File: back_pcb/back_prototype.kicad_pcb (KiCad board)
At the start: 2 copper layers, 40 x 100 mm, 358 parts

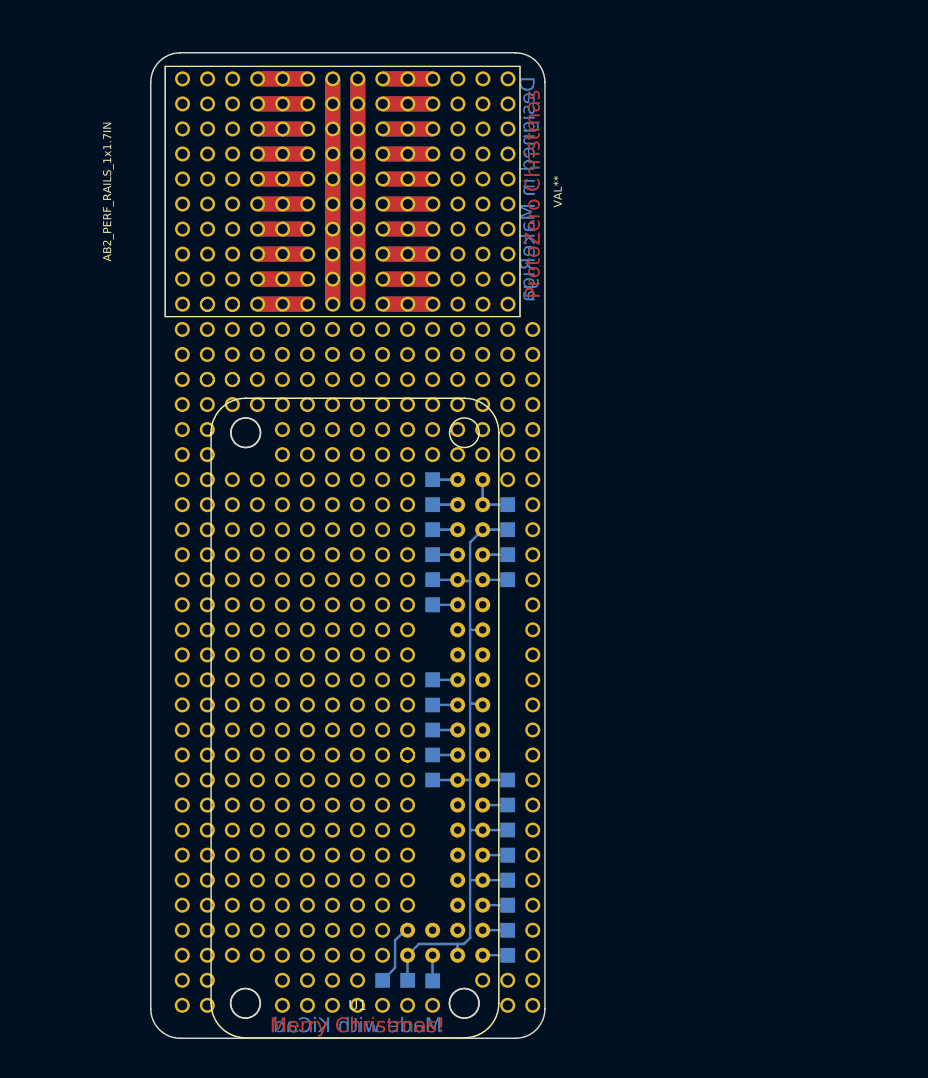
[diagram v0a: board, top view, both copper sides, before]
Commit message: Started new back PCB
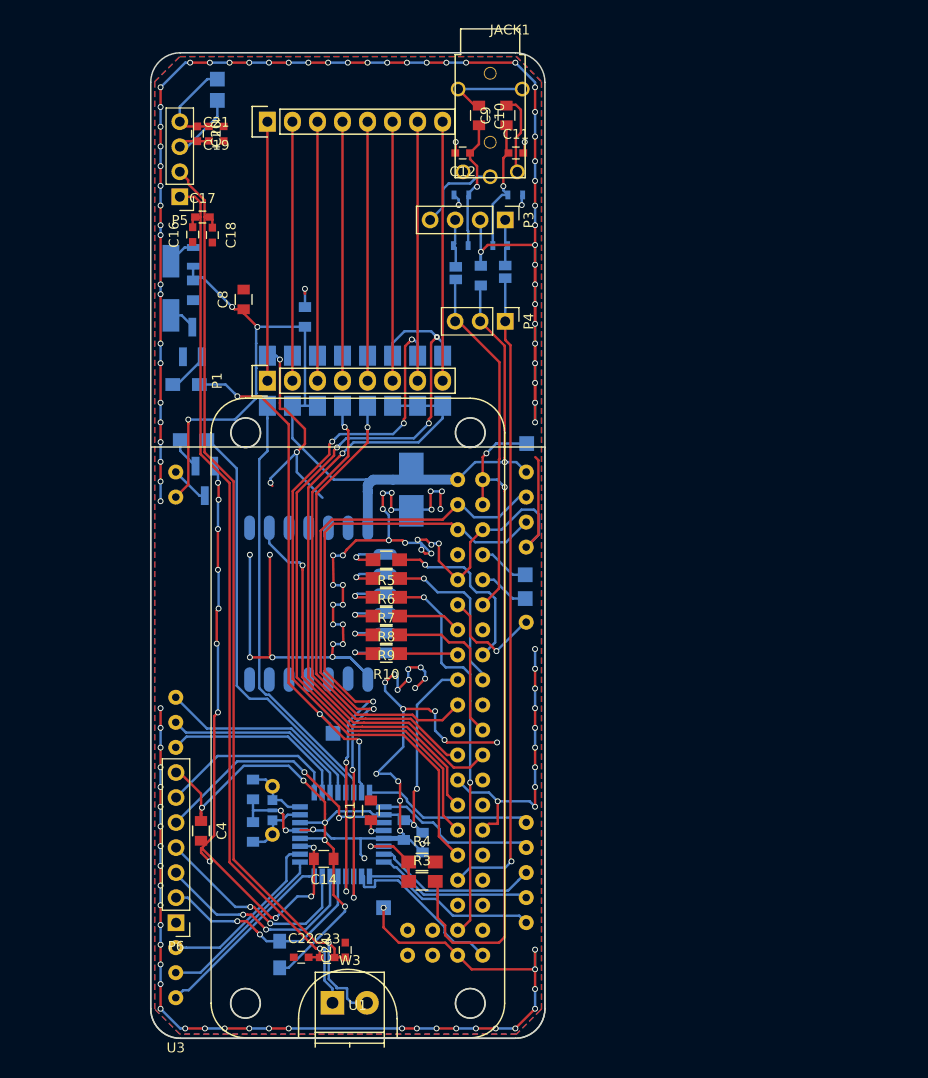
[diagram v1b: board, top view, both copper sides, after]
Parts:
- removed ? (x330): , single_proto_pad:PROTO_PAD
- removed AB2_PERF_RAILS_1x1.7IN: VAL**, prototyping_area_10x14:PROTO_AREA_10x14
- removed W10: RXD, Measurement_Points:Measurement_Point_Square-SMD-Pad_Small
- removed W13: SDA, Measurement_Points:Measurement_Point_Square-SMD-Pad_Small
- removed W14: SCL, Measurement_Points:Measurement_Point_Square-SMD-Pad_Small
- removed W15: MOSI, Measurement_Points:Measurement_Point_Square-SMD-Pad_Small
- removed W16: MISO, Measurement_Points:Measurement_Point_Square-SMD-Pad_Small
- removed W17: SCK, Measurement_Points:Measurement_Point_Square-SMD-Pad_Small
- removed W18: , Measurement_Points:Measurement_Point_Square-SMD-Pad_Small
- removed W19: CS1, Measurement_Points:Measurement_Point_Square-SMD-Pad_Small
- removed W20: GP4, Measurement_Points:Measurement_Point_Square-SMD-Pad_Small
- removed W21: GP17, Measurement_Points:Measurement_Point_Square-SMD-Pad_Small
- removed W22: GP12, Measurement_Points:Measurement_Point_Square-SMD-Pad_Small
- removed W23: GP16, Measurement_Points:Measurement_Point_Square-SMD-Pad_Small
- removed W24: GP20, Measurement_Points:Measurement_Point_Square-SMD-Pad_Small
- removed W25: GP21, Measurement_Points:Measurement_Point_Square-SMD-Pad_Small
- removed W26, W6, W8: GND, Measurement_Points:Measurement_Point_Square-SMD-Pad_Small
- removed W9: TXD, Measurement_Points:Measurement_Point_Square-SMD-Pad_Small
- added C1: C_Small, Capacitors_SMD:C_0805, F.Cu at (63.8, 116.9)
- added C10: C_Small, Capacitors_SMD:C_0805, F.Cu at (74.8, 46.4)
- added C11: C_Small, Capacitors_SMD:C_0603, F.Cu at (78.5, 50.2)
- added C12: C, Capacitors_SMD:C_0603, F.Cu at (73.2, 50.2)
- added C13: C_Small, Capacitors_SMD:C_0805, B.Cu at (75.0, 62.6)
- added C14: C_Small, Capacitors_SMD:C_0805, F.Cu at (59.1, 121.8)
- added C15: C_Small, Capacitors_Tantalum_SMD:CP_Tantalum_Case-B_EIA-3528-21_Hand, B.Cu at (67.9, 84.3)
- added C16: C_Small, Capacitors_SMD:C_0603, F.Cu at (45.8, 58.4)
- added C17: C_Small, Capacitors_SMD:C_0603, F.Cu at (46.7, 56.7)
- added C18: C_Small, Capacitors_SMD:C_0603, F.Cu at (47.8, 58.5)
- added C19: C_Small, Capacitors_SMD:C_0603, F.Cu at (48.1, 47.5)
- added C2: C_Small, Capacitors_SMD:C_0805, B.Cu at (51.9, 119.1)
- added C20: C_Small, Capacitors_SMD:C_0603, F.Cu at (46.2, 48.2)
- added C21: C_Small, Capacitors_SMD:C_0603, F.Cu at (48.1, 48.9)
- added C22: C_Small, Capacitors_SMD:C_0603, F.Cu at (56.8, 131.8)
- added C23: C_Small, Capacitors_SMD:C_0603, F.Cu at (59.4, 131.8)
- added C24: C_Small, Capacitors_SMD:C_0603, F.Cu at (61.2, 131.0)
- added C25: C_Small, Capacitors_SMD:C_0805, B.Cu at (45.8, 64.1)
- added C3: C_Small, Capacitors_SMD:C_0805, B.Cu at (51.9, 114.7)
- added C4: C_Small, Capacitors_SMD:C_0805, F.Cu at (46.6, 119.0)
- added C5: C_Small, Capacitors_SMD:C_0805, B.Cu at (67.2, 118.9)
- added C6: C_Small, Capacitors_SMD:C_0805, B.Cu at (57.1, 66.8)
- added C7: C_Small, Capacitors_SMD:C_0805, B.Cu at (69.1, 120.1)
- added C8: C_Small, Capacitors_SMD:C_0805, F.Cu at (50.9, 65.0)
- added C9: C, Capacitors_SMD:C_0805, F.Cu at (77.6, 46.4)
- added D1: D, Diodes_SMD:MiniMELF_Handsoldering, B.Cu at (43.5, 63.9)
- added IC1: ATMEGA328P-A, Housings_QFP:TQFP-32_7x7mm_Pitch0.8mm, B.Cu at (60.9, 119.3)
- added JACK1: AB2_JACK_3.5MM-4P, footprints:4P_RPi_AV_jack, F.Cu at (75.9, 52.6)
- added JP1: JUMPER, Connect:GS2, B.Cu at (77.5, 62.2)
- added JP2: JUMPER, Connect:GS2, B.Cu at (72.5, 62.4)
- added P1: SwitchableHeader-3x08, switchable_header:Pin_Header_Straight_1x08, F.Cu at (53.3, 73.3)
- added P2: CONN_01X08, Pin_Headers:Pin_Header_Straight_1x08, F.Cu at (53.3, 47.0)
- added P3: CONN_01X04, Pin_Headers:Pin_Header_Straight_1x04_Pitch2.54mm, F.Cu at (77.5, 57.0)
- added P4: CONN_01X03, Pin_Headers:Pin_Header_Straight_1x03_Pitch2.54mm, F.Cu at (77.5, 67.2)
- added P5: CONN_01X04, Pin_Headers:Pin_Header_Straight_1x04_Pitch2.54mm, F.Cu at (44.5, 54.6)
- added P6: CONN_01X07, Pin_Headers:Pin_Header_Straight_1x07_Pitch2.54mm, F.Cu at (44.1, 128.3)
- added Q1: BC547, footprints:SOT-23_BC847B_Handsoldering, B.Cu at (45.7, 69.3)
- added Q2: BC547, footprints:SOT-23_BC847B_Handsoldering, B.Cu at (47.0, 83.4)
- added R1: R, Resistors_SMD:R_0603, B.Cu at (78.5, 54.4)
- added R10: R, Resistors_SMD:R_0805_HandSoldering, F.Cu at (65.4, 101.0)
- added R11: R, Resistors_SMD:R_0805_HandSoldering, B.Cu at (54.6, 131.5)
- added R12: R, Resistors_SMD:R_0805_HandSoldering, B.Cu at (45.1, 73.7)
- added R13: R, Resistors_SMD:R_0805_HandSoldering, B.Cu at (45.8, 79.2)
- added R14: R_Small, Resistors_SMD:R_0603, B.Cu at (77.0, 59.6)
- added R15: R_Small, Resistors_SMD:R_0603, B.Cu at (73.0, 59.6)
- added R16: R_Small, Resistors_SMD:R_0805, B.Cu at (45.8, 60.7)
- added R2: R_Small, Resistors_SMD:R_0603, B.Cu at (73.0, 54.4)
- added R3: R, Resistors_SMD:R_0805_HandSoldering, F.Cu at (69.0, 124.1)
- added R4: R, Resistors_SMD:R_0805_HandSoldering, F.Cu at (69.0, 122.1)
- added R5: R, Resistors_SMD:R_0805_HandSoldering, F.Cu at (65.4, 91.4)
- added R6: R, Resistors_SMD:R_0805_HandSoldering, F.Cu at (65.4, 93.3)
- added R7: R, Resistors_SMD:R_0805_HandSoldering, F.Cu at (65.4, 95.2)
- added R8: R, Resistors_SMD:R_0805_HandSoldering, F.Cu at (65.4, 97.2)
- added R9: R, Resistors_SMD:R_0805_HandSoldering, F.Cu at (65.4, 99.1)
- added U2: ESP-12E, ESP12E_SMD:ESP-12E_-1_-22, B.Cu at (49.5, 88.9)
- added U3: KEYPAD_OVERLAY, common-footprints:keypad_overlay, F.Cu at (41.5, 80.0)
- added X1: CRYSTAL_TH_SMD, footprints:Crystal_HC49_CSTCE, B.Cu at (53.8, 114.4)
- U1: value (none) -> Pi0Top; footprint Pi0Top:Pi0Top -> common-footprints:pi0outline
- W1: value 3V3 -> TEST_1P
- W11: value VBAT -> TEST_1P
- W12, W5, W7: value GND -> TEST_1P
- W2: value GP1 -> TEST_1P
- W3: value RST -> MIC; footprint Measurement_Points:Measurement_Point_Square-SMD-Pad_Small -> Terminal_Blocks:TerminalBlock_Pheonix_PT-3.5mm_2pol; moved to F.Cu
- W4: value TV_OUT -> TEST_1P
- moved W4 90.8 mm to (48.3, 44.8)
- moved W5 55.3 mm to (48.3, 42.7)
- moved U1 41.3 mm to (72.6, 83.3)
- moved W7 27.2 mm to (60.0, 109.0)
- moved W2 21.0 mm to (79.5, 95.4)
- moved W1 14.2 mm to (79.5, 93.0)
- moved W3 10.4 mm to (59.9, 136.4)
- moved W12 7.76 mm to (65.1, 126.7)
- moved W11 6.49 mm to (79.7, 79.7)
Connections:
- U1 pad 11: Net-(U1-Pad11) -> KEYPAD_GPIO
- U1 pad 12: Net-(U1-Pad12) -> AUDIO_0
- U1 pad 13: Net-(U1-Pad13) -> SD_D3
- U1 pad 15: Net-(U1-Pad15) -> SD_CLK
- U1 pad 16: Net-(U1-Pad16) -> SD_CMD
- U1 pad 18: Net-(U1-Pad18) -> SD_D0
- U1 pad 19: Net-(U1-Pad19) -> DI
- U1 pad 21: Net-(U1-Pad21) -> (no net)
- U1 pad 22: Net-(U1-Pad22) -> SD_D1
- U1 pad 23: Net-(U1-Pad23) -> SCK
- U1 pad 24: Net-(U1-Pad24) -> CS
- U1 pad 26: Net-(U1-Pad26) -> (no net)
- U1 pad 27: Net-(U1-Pad27) -> SD_RST
- U1 pad 28: Net-(U1-Pad28) -> (no net)
- U1 pad 29: Net-(U1-Pad29) -> DISPLAY_RST
- U1 pad 3: Net-(U1-Pad3) -> SDA
- U1 pad 31: Net-(U1-Pad31) -> DISPLAY_DC
- U1 pad 32: Net-(U1-Pad32) -> (no net)
- U1 pad 33: Net-(U1-Pad33) -> AUDIO_1
- U1 pad 35: Net-(U1-Pad35) -> (no net)
- U1 pad 36: Net-(U1-Pad36) -> (no net)
- U1 pad 37: Net-(U1-Pad37) -> SD_D2
- U1 pad 38: Net-(U1-Pad38) -> (no net)
- U1 pad 40: Net-(U1-Pad40) -> KEYPAD_INT
- U1 pad 41: Net-(U1-Pad41) -> (no net)
- U1 pad 42: Net-(U1-Pad42) -> (no net)
- U1 pad 43: Net-(U1-Pad43) -> (no net)
- U1 pad 44: GND -> (no net)
- U1 pad 5: Net-(U1-Pad5) -> SCL
- U1 pad 7: Net-(U1-Pad7) -> (no net)
- W1 pad 1: +3V3 -> Net-(U1-Pad8)
- W2 pad 1: Net-(U1-Pad28) -> Net-(U1-Pad10)
- W3 pad 1: Net-(U1-Pad42) -> Net-(C16-Pad2)
- W4 pad 1: Net-(U1-Pad43) -> Net-(C20-Pad2)
- W5 pad 1: GND -> Net-(C19-Pad2)
- W7 pad 1: GND -> VIBRO_PWM
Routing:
- net GND: track 73.1 -> 550.0 mm, vias 0 -> 167
- net +3V3: track 5.08 -> 192.4 mm, vias 0 -> 11
- net Net-(C17-Pad2): track 0.00 -> 99.0 mm, vias 0 -> 1
- net Net-(C16-Pad2): track 0.00 -> 93.3 mm, vias 0 -> 1
- net DISPLAY_RST: track 0.00 -> 79.2 mm, vias 0 -> 3
- net DISPLAY_DC: track 0.00 -> 73.6 mm, vias 0 -> 3
- net SDA: track 0.00 -> 67.1 mm, vias 0 -> 3
- net AUDIO_1: track 0.00 -> 65.8 mm, vias 0 -> 1
- net VPP: track 5.08 -> 70.7 mm, vias 0 -> 2
- net SCL: track 0.00 -> 64.9 mm, vias 0 -> 3
- net CS: track 0.00 -> 64.2 mm, vias 0 -> 1
- net VIBRO_PWM: track 0.00 -> 54.4 mm, vias 0 -> 3
- net SCK: track 0.00 -> 47.2 mm, vias 0 -> 1
- net DI: track 0.00 -> 46.8 mm, vias 0 -> 1
- net DISPLAY_BL: track 0.00 -> 43.7 mm
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- added copper zone on B.Cu, net GND
- added copper zone on F.Cu, net GND
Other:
- outline, holes or cut-outs redrawn
- net class Default: clearance 0.2 -> 0.16
- rule trace_clearance: 0.2 -> 0.16
- rule via_min_drill: 0.3 -> 0.25
- board text removed: "Designed in MakeRiga"
- board text removed: "Made with KiCad"
- board text removed: "Merry Christmas!"
- board text removed: "ProtoZero Christmas"

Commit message: Back board almost finished
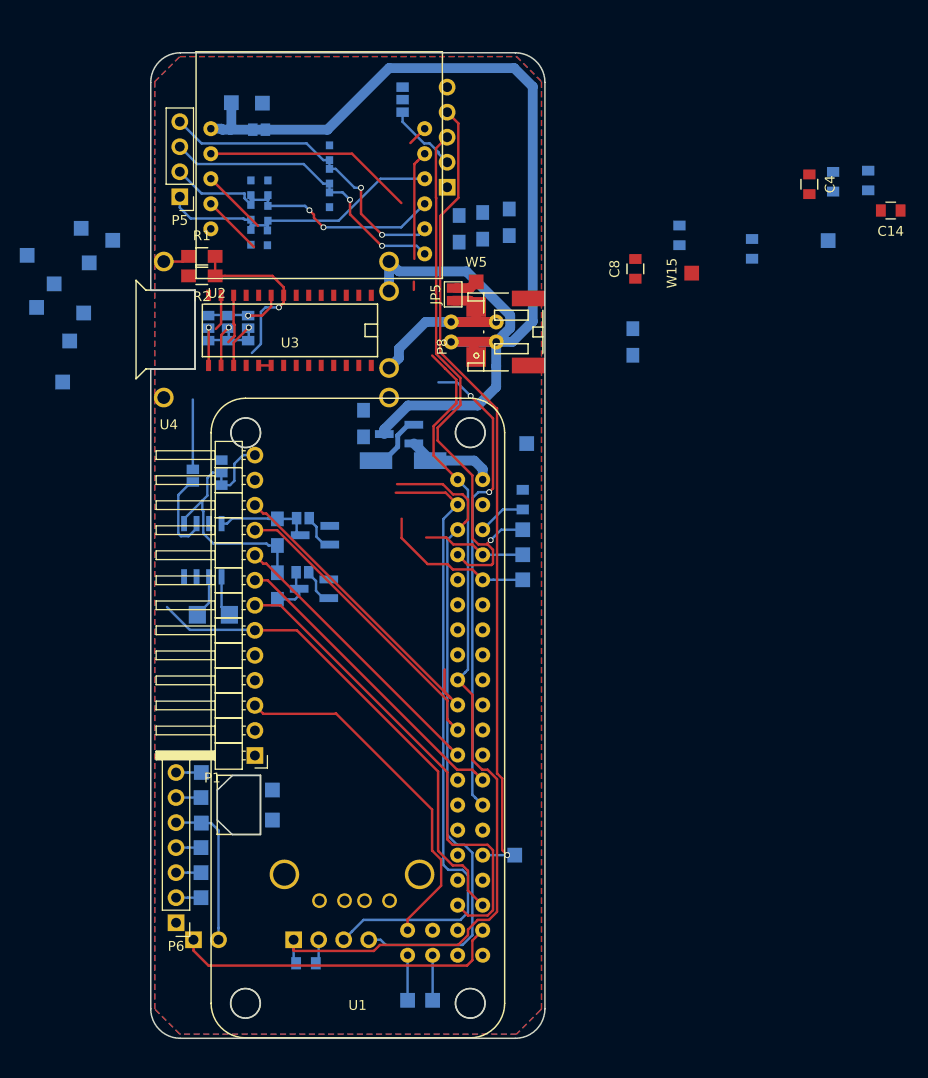
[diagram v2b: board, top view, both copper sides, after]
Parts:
- removed C1, C10, C2, C3: C_Small, Capacitors_SMD:C_0805
- removed C11: C_Small, Capacitors_SMD:C_0603
- removed C12: C, Capacitors_SMD:C_0603
- removed C9: C, Capacitors_SMD:C_0805
- removed IC1: ATMEGA328P-A, Housings_QFP:TQFP-32_7x7mm_Pitch0.8mm
- removed JACK1: AB2_JACK_3.5MM-4P, footprints:4P_RPi_AV_jack
- removed R10, R11, R12, R13: R, Resistors_SMD:R_0805_HandSoldering
- removed R14, R15: R_Small, Resistors_SMD:R_0603
- removed R16: R_Small, Resistors_SMD:R_0805
- removed X1: CRYSTAL_TH_SMD, footprints:Crystal_HC49_CSTCE
- added JP10: Jumper_NC_Small, Connect:GS2, B.Cu at (56.9, 87.2)
- added JP3: JUMPER3, Connect:GS3, B.Cu at (47.3, 67.9)
- added JP4: JUMPER3, Connect:GS3, B.Cu at (51.4, 67.9)
- added JP5: JUMPER, Connect:GS2, F.Cu at (72.2, 64.5)
- added JP6: JUMPER3, Connect:GS3, B.Cu at (49.4, 67.9)
- added JP7: JUMPER3, Connect:GS3, B.Cu at (48.7, 82.6)
- added JP8: JUMPER3, Connect:GS3, B.Cu at (67.1, 44.8)
- added JP9: Jumper_NC_Small, Connect:GS2, B.Cu at (56.9, 92.7)
- added P7: EXPANSION_BOTTOM2, Pin_Headers:Pin_Header_Angled_1x02_Pitch2.54mm, B.Cu at (45.8, 130.0)
- added P8: CONN_01X02, footprints:JST_PH_S2B-PH-SM4-TB_02x2.00mm_Angled, F.Cu at (77.1, 68.3)
- added Q3: Q_NMOS_GSD, TO_SOT_Packages_SMD:SOT-23_Handsoldering, B.Cu at (58.2, 89.0)
- added U4: TP4056_BREAKOUT, footprints:TP4056_BREAKOUT, F.Cu at (54.5, 68.1)
- added U5: RTC, Housings_SOIC:SOIC-8_3.9x4.9mm_Pitch1.27mm, B.Cu at (46.8, 90.5)
- added W10: TEST_1P, Measurement_Points:Measurement_Point_Square-SMD-Pad_Small, B.Cu at (46.6, 123.2)
- added W13: TEST_1P, Measurement_Points:Measurement_Point_Square-SMD-Pad_Small, B.Cu at (46.6, 125.7)
- added W14: TEST_1P, Measurement_Points:Measurement_Point_Square-SMD-Pad_Small, B.Cu at (52.8, 45.1)
- added W15: BAT-, Measurement_Points:Measurement_Point_Square-SMD-Pad_Small, F.Cu at (96.4, 62.4)
- added W16: BAT+, Measurement_Points:Measurement_Point_Square-SMD-Pad_Small, B.Cu at (49.7, 45.1)
- added W17: TEST_1P, Measurement_Points:Measurement_Point_Square-SMD-Pad_Small, B.Cu at (37.6, 59.0)
- added W18: TEST_1P, Measurement_Points:Measurement_Point_Square-SMD-Pad_Small, B.Cu at (34.7, 66.4)
- added W19: TEST_1P, Measurement_Points:Measurement_Point_Square-SMD-Pad_Small, B.Cu at (29.9, 65.8)
- added W20: TEST_1P, Measurement_Points:Measurement_Point_Square-SMD-Pad_Small, B.Cu at (32.6, 73.4)
- added W21: TEST_1P, Measurement_Points:Measurement_Point_Square-SMD-Pad_Small, B.Cu at (31.7, 63.4)
- added W22: TEST_1P, Measurement_Points:Measurement_Point_Square-SMD-Pad_Small, B.Cu at (34.4, 57.8)
- added W23: TEST_1P, Measurement_Points:Measurement_Point_Square-SMD-Pad_Small, B.Cu at (29.0, 60.6)
- added W24: TEST_1P, Measurement_Points:Measurement_Point_Square-SMD-Pad_Small, B.Cu at (35.3, 61.3)
- added W25: TEST_1P, Measurement_Points:Measurement_Point_Square-SMD-Pad_Small, B.Cu at (53.8, 114.8)
- added W26: TEST_1P, Measurement_Points:Measurement_Point_Square-SMD-Pad_Small, B.Cu at (53.8, 117.9)
- added W27: TEST_1P, Measurement_Points:Measurement_Point_Square-SMD-Pad_Small, B.Cu at (46.6, 113.0)
- added W28: TEST_1P, Measurement_Points:Measurement_Point_Square-SMD-Pad_Small, B.Cu at (33.3, 69.2)
- added W29: TEST_1P, Measurement_Points:Measurement_Point_Square-SMD-Pad_Small, B.Cu at (46.6, 118.2)
- added W6: TEST_1P, Measurement_Points:Measurement_Point_Square-SMD-Pad_Small, B.Cu at (79.2, 88.4)
- added W8: TEST_1P, Measurement_Points:Measurement_Point_Square-SMD-Pad_Small, B.Cu at (46.6, 115.6)
- added W9: TEST_1P, Measurement_Points:Measurement_Point_Square-SMD-Pad_Small, B.Cu at (46.6, 120.7)
- added Y1: Crystal_Small, Crystals:Crystal_SMD_G8-2pin_3.2x1.5mm_HandSoldering, B.Cu at (47.9, 97.0)
- C15: footprint Capacitors_Tantalum_SMD:CP_Tantalum_Case-B_EIA-3528-21_Hand -> Capacitors_SMD:C_0805
- C16, C17, C18, C19, C20, C21, C22, C23, C24, R3, R4, R5, R6, R7, R8, R9: moved to B.Cu
- D1: value D -> D_Small; footprint Diodes_SMD:MiniMELF_Handsoldering -> Diodes_SMD:D_MiniMELF_Handsoldering
- P1: value SwitchableHeader-3x08 -> EXPANSION_LEFT; footprint switchable_header:Pin_Header_Straight_1x08 -> Pin_Headers:Pin_Header_Angled_1x13_Pitch2.54mm
- P2: value CONN_01X08 -> EXPANSION_BOTTOM; footprint Pin_Headers:Pin_Header_Straight_1x08 -> Pin_Headers:Pin_Header_Angled_1x04_Pitch2.54mm; moved to B.Cu
- P3: value CONN_01X04 -> EXPANSION_TOP; footprint Pin_Headers:Pin_Header_Straight_1x04_Pitch2.54mm -> Pin_Headers:Pin_Header_Angled_1x05_Pitch2.54mm; moved to B.Cu
- P4: value CONN_01X03 -> USB_A; footprint Pin_Headers:Pin_Header_Straight_1x03_Pitch2.54mm -> Connect:USB_A; moved to B.Cu
- P6: value CONN_01X07 -> ATMEGA_HEADER
- Q1: value BC547 -> Q_PMOS_GSD; footprint footprints:SOT-23_BC847B_Handsoldering -> TO_SOT_Packages_SMD:SOT-23_Handsoldering
- Q2: value BC547 -> Q_NMOS_GSD; footprint footprints:SOT-23_BC847B_Handsoldering -> TO_SOT_Packages_SMD:SOT-23_Handsoldering
- R1: footprint Resistors_SMD:R_0603 -> Resistors_SMD:R_0805_HandSoldering; moved to F.Cu
- R2: value R_Small -> R; footprint Resistors_SMD:R_0603 -> Resistors_SMD:R_0805_HandSoldering; moved to F.Cu
- U1: value Pi0Top -> PI ZERO
- U2: value ESP-12E -> SIM800_BREAKOUT; footprint ESP12E_SMD:ESP-12E_-1_-22 -> footprints:SIM800_BREAKOUT; moved to F.Cu
- U3: value KEYPAD_OVERLAY -> MCP23017; footprint common-footprints:keypad_overlay -> SMD_Packages:SOIC-28
- W11: value TEST_1P -> BAT_IN
- W3: value MIC -> TEST_1P; footprint Terminal_Blocks:TerminalBlock_Pheonix_PT-3.5mm_2pol -> Measurement_Points:Measurement_Point_Square-SMD-Pad_Small; moved to B.Cu
- W5: moved to F.Cu
- moved W4 93.3 mm to (67.6, 136.1)
- moved C4 90.1 mm to (108.3, 53.3)
- moved C14 87.4 mm to (116.6, 56.0)
- moved P2 83.1 mm to (56.0, 130.0), turned to 270 degrees
- moved W12 81.3 mm to (110.2, 59.1)
- moved C7 81.0 mm to (114.3, 53.0)
- moved C5 78.9 mm to (110.7, 53.1)
- moved C24 77.9 mm to (51.7, 53.7)
- moved C23 76.0 mm to (51.7, 56.2), turned to 90 degrees
- moved C22 73.2 mm to (51.7, 58.7), turned to 90 degrees
- moved C25 69.2 mm to (57.3, 132.4), turned to 0 degrees
- moved P4 61.7 mm to (58.6, 126.0), turned to 0 degrees
- moved R4 56.9 mm to (90.4, 69.3), turned to 270 degrees
- moved R3 46.8 mm to (63.1, 77.6), turned to 90 degrees
- moved C8 39.9 mm to (90.7, 61.9)
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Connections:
- C16 pad 2: Net-(C16-Pad2) -> MIC+
- C17 pad 1: Net-(C16-Pad2) -> MIC+
- C17 pad 2: Net-(C17-Pad2) -> MIC-
- C18 pad 1: Net-(C17-Pad2) -> MIC-
- C19 pad 2: Net-(C19-Pad2) -> SPK+
- C20 pad 1: Net-(C19-Pad2) -> SPK+
- C20 pad 2: Net-(C20-Pad2) -> SPK-
- C21 pad 1: Net-(C20-Pad2) -> SPK-
- C22 pad 2: Net-(C16-Pad2) -> MIC+
- C23 pad 1: Net-(C16-Pad2) -> MIC+
- C23 pad 2: Net-(C17-Pad2) -> MIC-
- C24 pad 1: Net-(C17-Pad2) -> MIC-
- D1 pad 1: Net-(D1-Pad1) -> VPP
- D1 pad 2: Net-(D1-Pad2) -> VDD
- JP1 pad 1: Net-(JP1-Pad1) -> +BATT
- JP1 pad 2: AUDIO_1 -> +BATT
- JP2 pad 1: AUDIO_0 -> RTC_ALARM
- P1 pad 1: DISPLAY_BL -> +BATT
- P1 pad 10: SCK -> MISO
- P1 pad 11: Net-(P1-Pad11) -> MOSI
- P1 pad 12: (no net) -> GND
- P1 pad 13: DI -> +3V3
- P1 pad 2: Net-(P1-Pad2) -> +5V
- P1 pad 3: GND -> TV_OUT
- P1 pad 4: +3V3 -> GND
- P1 pad 5: Net-(P1-Pad5) -> VDD
- P1 pad 6: GND -> LH_GPIO_2
- P1 pad 7: +3V3 -> LH_GPIO_1
- P1 pad 8: Net-(P1-Pad8) -> CS
- P1 pad 9: GND -> SCK
- P2 pad 1: Net-(P1-Pad2) -> +3V3
- P2 pad 2: Net-(P1-Pad5) -> GND
- P2 pad 3: Net-(P1-Pad8) -> SDA
- P2 pad 4: Net-(P1-Pad11) -> SCL
- P3 pad 1: Net-(JP1-Pad1) -> +5V
- P3 pad 2: GND -> +3V3
- P3 pad 3: Net-(JP2-Pad2) -> IR_TX
- P3 pad 4: MIC -> IR_RX
- P4 pad 1: AUDIO_1 -> +5V
- P4 pad 2: +3V3 -> USB_D-
- P4 pad 3: AUDIO_0 -> USB_D+
- P5 pad 1: Net-(C16-Pad2) -> MIC+
- P5 pad 2: Net-(C17-Pad2) -> MIC-
- P5 pad 3: Net-(C20-Pad2) -> SPK-
- P5 pad 4: Net-(C19-Pad2) -> SPK+
- P6 pad 7: +3V3 -> Net-(P6-Pad7)
- Q1 pad 1: Net-(D1-Pad2) -> VDD
- Q1 pad 2: Net-(Q1-Pad2) -> VPP
- Q1 pad 3: GND -> +BATT
- Q2 pad 1: KEYPAD_BL- -> GND
- Q2 pad 2: Net-(Q2-Pad2) -> SCL
- Q2 pad 3: GND -> Net-(JP9-Pad1)
- R1 pad 1: Net-(C11-Pad1) -> VDD
- R1 pad 2: GND -> CHARGING_SENSE
- R2 pad 1: GND -> CHARGING_SENSE
- R2 pad 2: Net-(C10-Pad2) -> GND
- R3 pad 1: Net-(IC1-Pad22) -> VDD
- R3 pad 2: VPP -> GND
- R4 pad 1: Net-(IC1-Pad22) -> (no net)
- R4 pad 2: GND -> FLASH_LED
- R5 pad 1: SD_CMD -> (no net)
- R5 pad 2: Net-(R5-Pad2) -> NOTIF_LED_R
- R6 pad 1: SD_D0 -> (no net)
- R6 pad 2: Net-(R6-Pad2) -> NOTIF_LED_G
- R7 pad 1: SD_D2 -> (no net)
- R7 pad 2: Net-(R7-Pad2) -> NOTIF_LED_B
- R8 pad 1: SD_D3 -> +3V3
- R8 pad 2: Net-(R8-Pad2) -> Net-(JP9-Pad1)
- R9 pad 1: SD_D1 -> Net-(JP10-Pad1)
- R9 pad 2: Net-(R9-Pad2) -> +3V3
- U1 pad 10: Net-(U1-Pad10) -> SIM800_TXD
- U1 pad 11: KEYPAD_GPIO -> (no net)
- U1 pad 12: AUDIO_0 -> (no net)
- U1 pad 13: SD_D3 -> (no net)
- U1 pad 15: SD_CLK -> (no net)
- U1 pad 16: SD_CMD -> (no net)
- U1 pad 18: SD_D0 -> (no net)
- U1 pad 19: DI -> MOSI
- U1 pad 21: (no net) -> MISO
- U1 pad 22: SD_D1 -> (no net)
- U1 pad 24: CS -> (no net)
- U1 pad 26: (no net) -> CS
- U1 pad 27: SD_RST -> (no net)
- U1 pad 28: (no net) -> MCP_INT
- U1 pad 29: DISPLAY_RST -> (no net)
- U1 pad 31: DISPLAY_DC -> (no net)
- U1 pad 32: (no net) -> IR_RX
- U1 pad 33: AUDIO_1 -> (no net)
- U1 pad 35: (no net) -> LH_GPIO_1
- U1 pad 36: (no net) -> LH_GPIO_2
- U1 pad 37: SD_D2 -> (no net)
- U1 pad 38: (no net) -> BH_GPIO
- U1 pad 40: KEYPAD_INT -> (no net)
- U1 pad 42: (no net) -> PI_RST
- U1 pad 43: (no net) -> TV_OUT
- U1 pad 44: (no net) -> Net-(U1-Pad44)
- U1 pad 7: (no net) -> IR_TX
- U1 pad 8: Net-(U1-Pad8) -> SIM800_RXD
- U2 pad 10: Net-(R6-Pad2) -> SPK+
- U2 pad 11: Net-(R7-Pad2) -> SPK-
- U2 pad 2: (no net) -> SIM800_RST
- U2 pad 3: SD_RST -> SIM800_RXD
- U2 pad 4: (no net) -> SIM800_TXD
- U2 pad 5: (no net) -> GND
- U2 pad 6: (no net) -> SIM800_RING
- U2 pad 7: (no net) -> SIM800_DTR
- U2 pad 8: +3V3 -> MIC+
- U2 pad 9: Net-(R5-Pad2) -> MIC-
- U3 pad 1: ROW5 -> SIM800_DTR
- U3 pad 10: COL5 -> GND
- U3 pad 11: COL6 -> (no net)
- U3 pad 12: +3V3 -> SCL
- U3 pad 13: KEYPAD_BL- -> SDA
- U3 pad 14: +3V3 -> (no net)
- U3 pad 15: SDA -> GND
- U3 pad 16: SCL -> GND
- U3 pad 18: KEYPAD_GPIO -> (no net)
- U3 pad 2: ROW4 -> SIM800_RING
- U3 pad 3: ROW3 -> SIM800_RST
- U3 pad 4: ROW2 -> (no net)
- U3 pad 5: ROW1 -> (no net)
- U3 pad 6: COL1 -> (no net)
- U3 pad 7: COL2 -> Net-(JP2-Pad2)
- U3 pad 8: COL3 -> CHARGING_SENSE
- U3 pad 9: COL4 -> +3V3
- W1 pad 1: Net-(U1-Pad8) -> SIM800_RXD
- W11 pad 1: VPP -> +BATT
- W2 pad 1: Net-(U1-Pad10) -> SIM800_TXD
- W3 pad 1: Net-(C16-Pad2) -> PI_RST
- W4 pad 1: Net-(C20-Pad2) -> Net-(U1-Pad44)
- W5 pad 1: Net-(C19-Pad2) -> GND
- W7 pad 1: VIBRO_PWM -> IR_RX
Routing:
- net GND: track 550.0 -> 30.0 mm, vias 167 -> 3
- net +BATT: track 0.00 -> 112.5 mm
- net Net-(C17-Pad2): track 99.0 -> 0.00 mm, vias 1 -> 0
- net Net-(C16-Pad2): track 93.3 -> 0.00 mm, vias 1 -> 0
- net IR_RX: track 0.00 -> 82.7 mm, vias 0 -> 1
- net DISPLAY_RST: track 79.2 -> 0.00 mm, vias 3 -> 0
- net DISPLAY_DC: track 73.6 -> 0.00 mm, vias 3 -> 0
- net AUDIO_1: track 65.8 -> 0.00 mm, vias 1 -> 0
- net VPP: track 70.7 -> 9.19 mm, vias 2 -> 0
- net +3V3: track 192.4 -> 132.4 mm, vias 11 -> 1
- net IR_TX: track 0.00 -> 56.9 mm, vias 0 -> 1
- net VIBRO_PWM: track 54.4 -> 0.00 mm, vias 3 -> 0
- net LH_GPIO_2: track 0.00 -> 50.4 mm
- net MCP_INT: track 0.00 -> 49.5 mm, vias 0 -> 2
- net LH_GPIO_1: track 0.00 -> 48.8 mm
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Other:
- outline, holes or cut-outs redrawn
